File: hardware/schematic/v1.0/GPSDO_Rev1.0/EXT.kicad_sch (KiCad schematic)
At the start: 12 parts, among them J1 Conn_Coaxial, J2 Conn_Coaxial, U12 BUF602IDBVT, U4 BUF602IDBVT

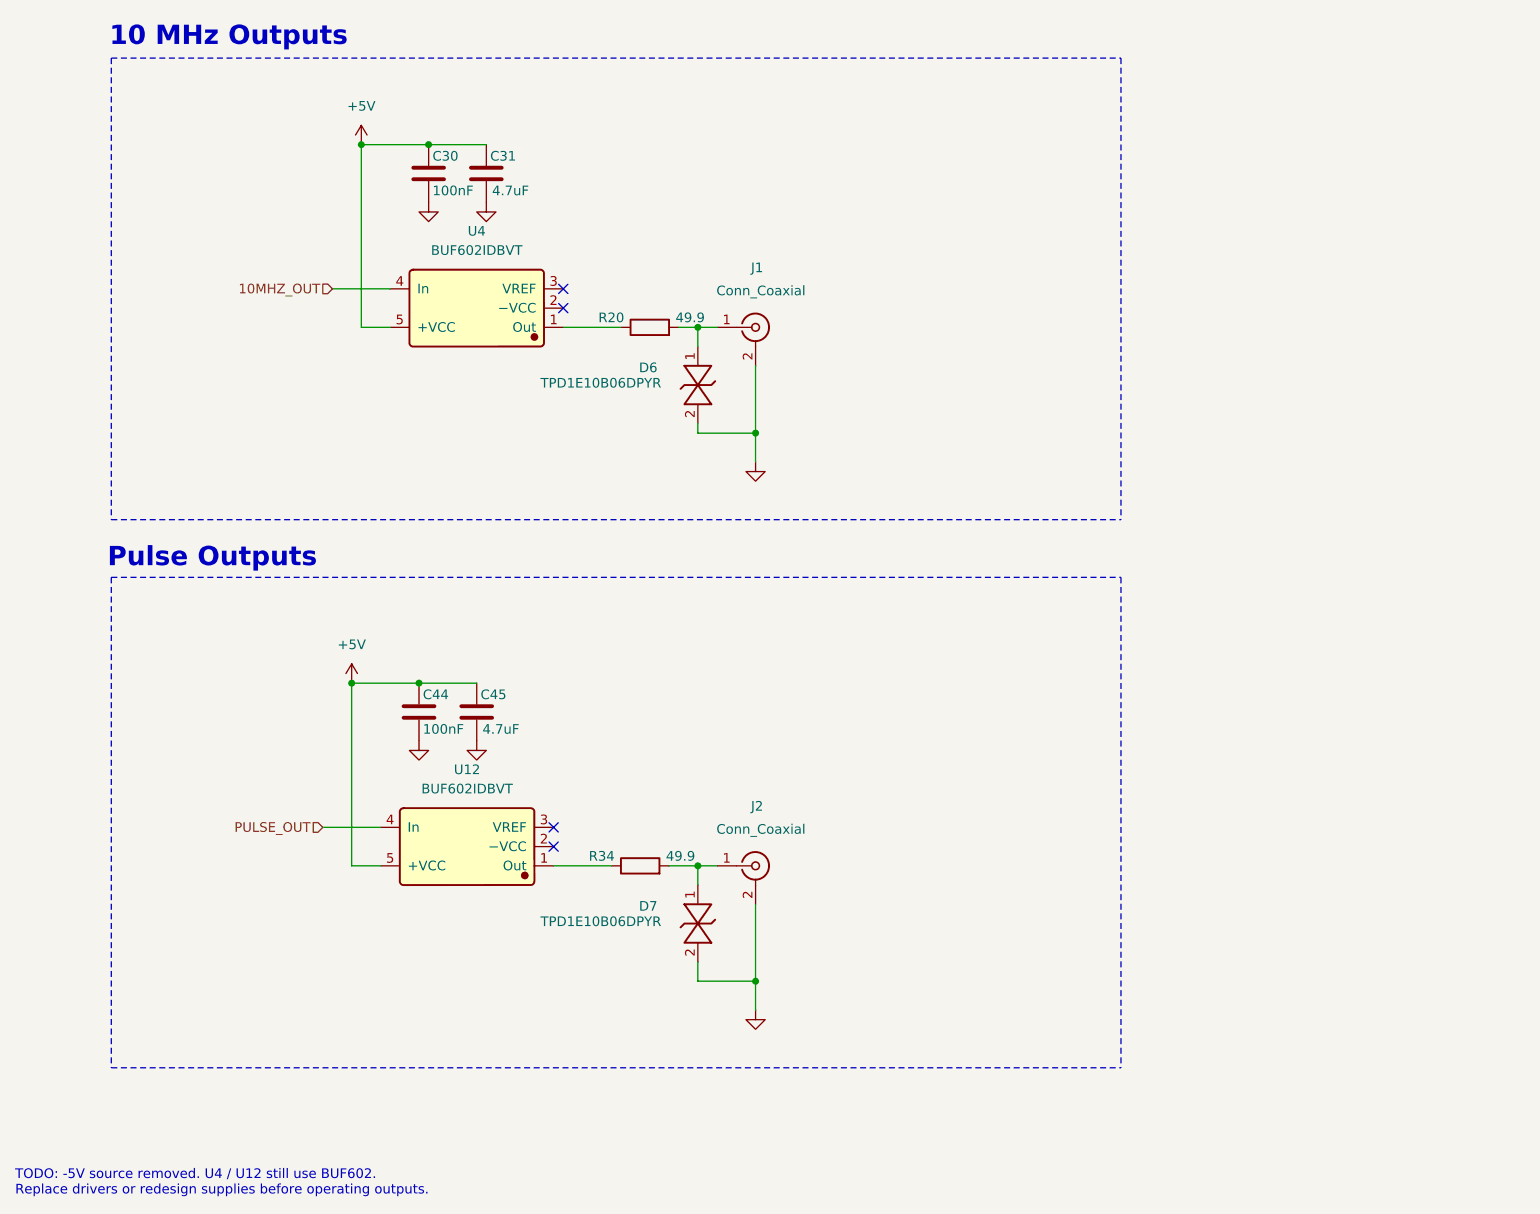
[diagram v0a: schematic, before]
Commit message: sch update
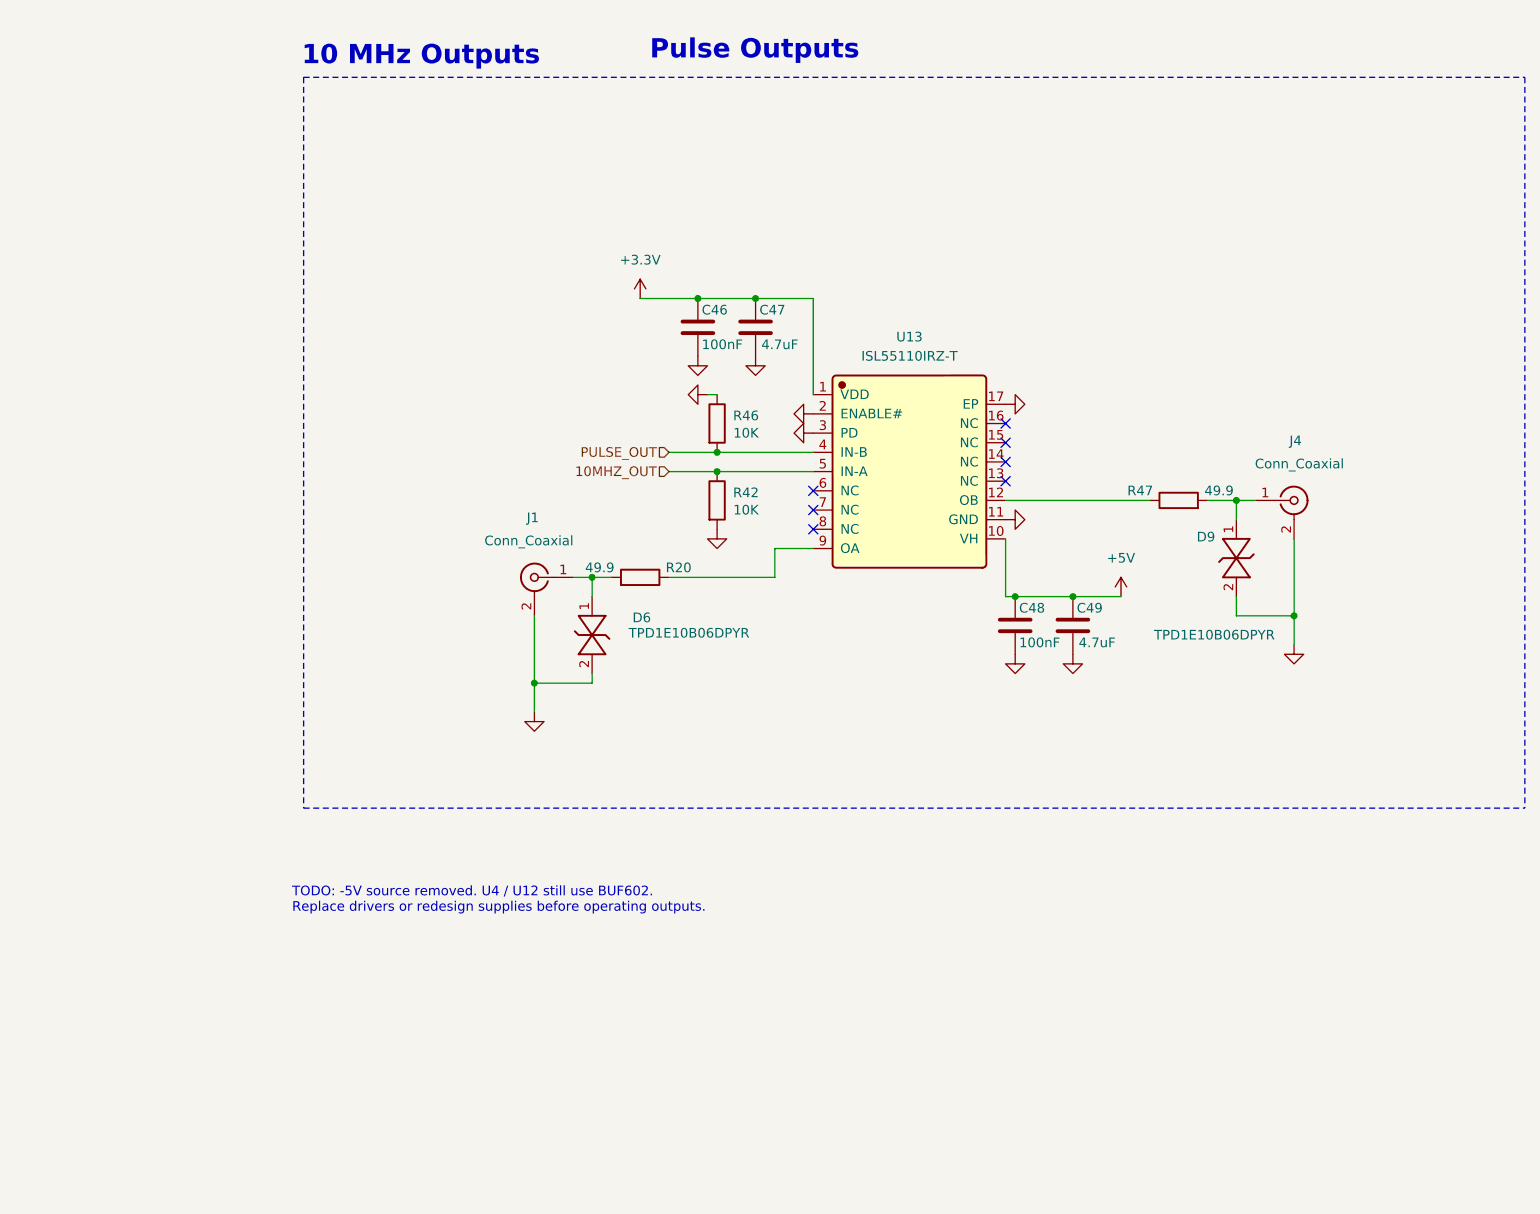
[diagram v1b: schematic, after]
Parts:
- removed C30, C44: 100nF, GPSDO_Rev1.0:C_0402_1005Metric, symbol GPSDO_Rev1.0:C__C_0402_1005Metric
- removed C31, C45: 4.7uF, GPSDO_Rev1.0:C_0603_1608Metric, symbol GPSDO_Rev1.0:C
- removed D7: TPD1E10B06DPYR, GPSDO_Rev1.0:TPD1E10B06DPYR, symbol GPSDO_Rev1.0:TPD1E10B06DPYR
- removed J2: Conn_Coaxial, GPSDO_Rev1.0:SMA_Amphenol_132289_EdgeMount, symbol GPSDO_Rev1.0:Conn_Coaxial
- removed R34: 49.9, GPSDO_Rev1.0:C_0603_1608Metric, symbol GPSDO_Rev1.0:R__C_0603_1608Metric
- removed U12, U4: BUF602IDBVT, GPSDO_Rev1.0:BUF602IDBVT, symbol GPSDO_Rev1.0:BUF602IDBVT
- added C46, C48: 100nF, GPSDO_Rev1.0:C_0402_1005Metric, symbol GPSDO_Rev1.0:C__C_0402_1005Metric
- added C47, C49: 4.7uF, GPSDO_Rev1.0:C_0603_1608Metric, symbol GPSDO_Rev1.0:C
- added D9: TPD1E10B06DPYR, GPSDO_Rev1.0:TPD1E10B06DPYR, symbol GPSDO_Rev1.0:TPD1E10B06DPYR
- added J4: Conn_Coaxial, GPSDO_Rev1.0:SMA_Amphenol_132289_EdgeMount, symbol GPSDO_Rev1.0:Conn_Coaxial
- added R42, R46: 10K, GPSDO_Rev1.0:R_0402_1005Metric, symbol GPSDO_Rev1.0:R__R_0402_1005Metric
- added R47: 49.9, GPSDO_Rev1.0:C_0603_1608Metric, symbol GPSDO_Rev1.0:R__C_0603_1608Metric
- added U13: ISL55110IRZ-T, GPSDO_Rev1.0:ISL55110IRZ-T, symbol GPSDO_Rev1.0:ISL55110IRZ-T
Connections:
- net +5V: now also C48.1, C49.1, U13.10 (VH)
- net 10MHZ_OUT: now also R42.1, U13.5 (IN-A)
- net GND: now also C46.2, C47.2, C48.2, C49.2, D9.2, J4.2 (Ext), R42.2, R46.1, U13.11 (GND), U13.17 (EP), U13.2 (ENABLE#), U13.3 (PD)
- net PULSE_OUT: now also R46.2, U13.4 (IN-B)
- net at R20.1: now also U13.9 (OA)
- new net: R47.1, U13.12 (OB)
- new net: D9.1, J4.1 (In), R47.2
- new net +3.3V: C46.1, C47.1, U13.1 (VDD)
- no-connect marks 4 -> 7
